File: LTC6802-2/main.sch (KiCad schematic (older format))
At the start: 10 parts, among them P1 CONN_01X13, P2 CONN_01X04, P3 CONN_01X04, P4 CONN_01X06, P5 CONN_01X13, U1 LTC6802-2

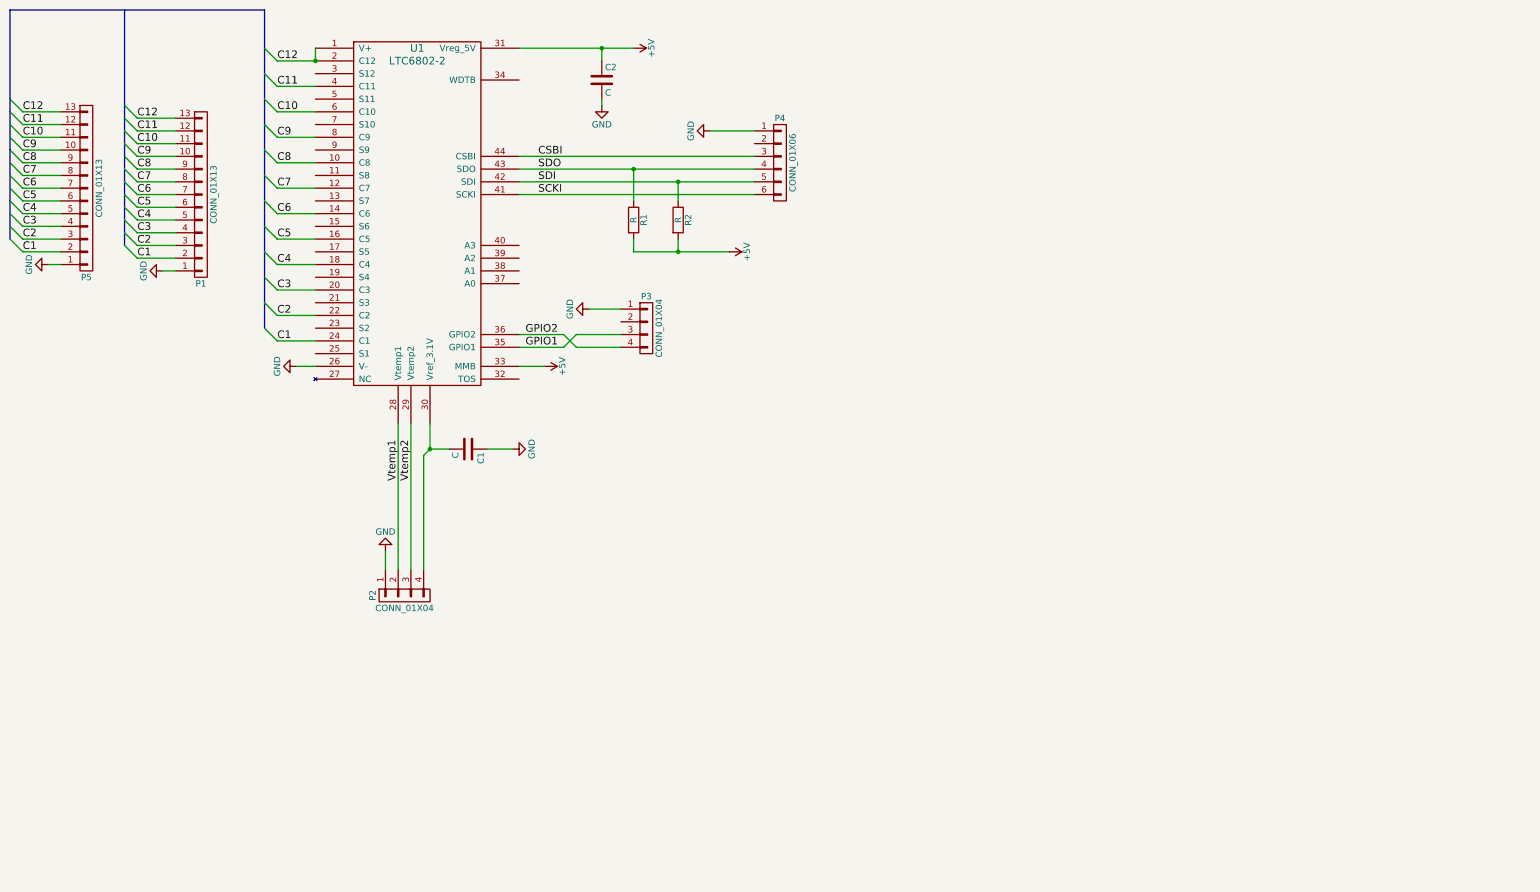
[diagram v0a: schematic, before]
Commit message: test
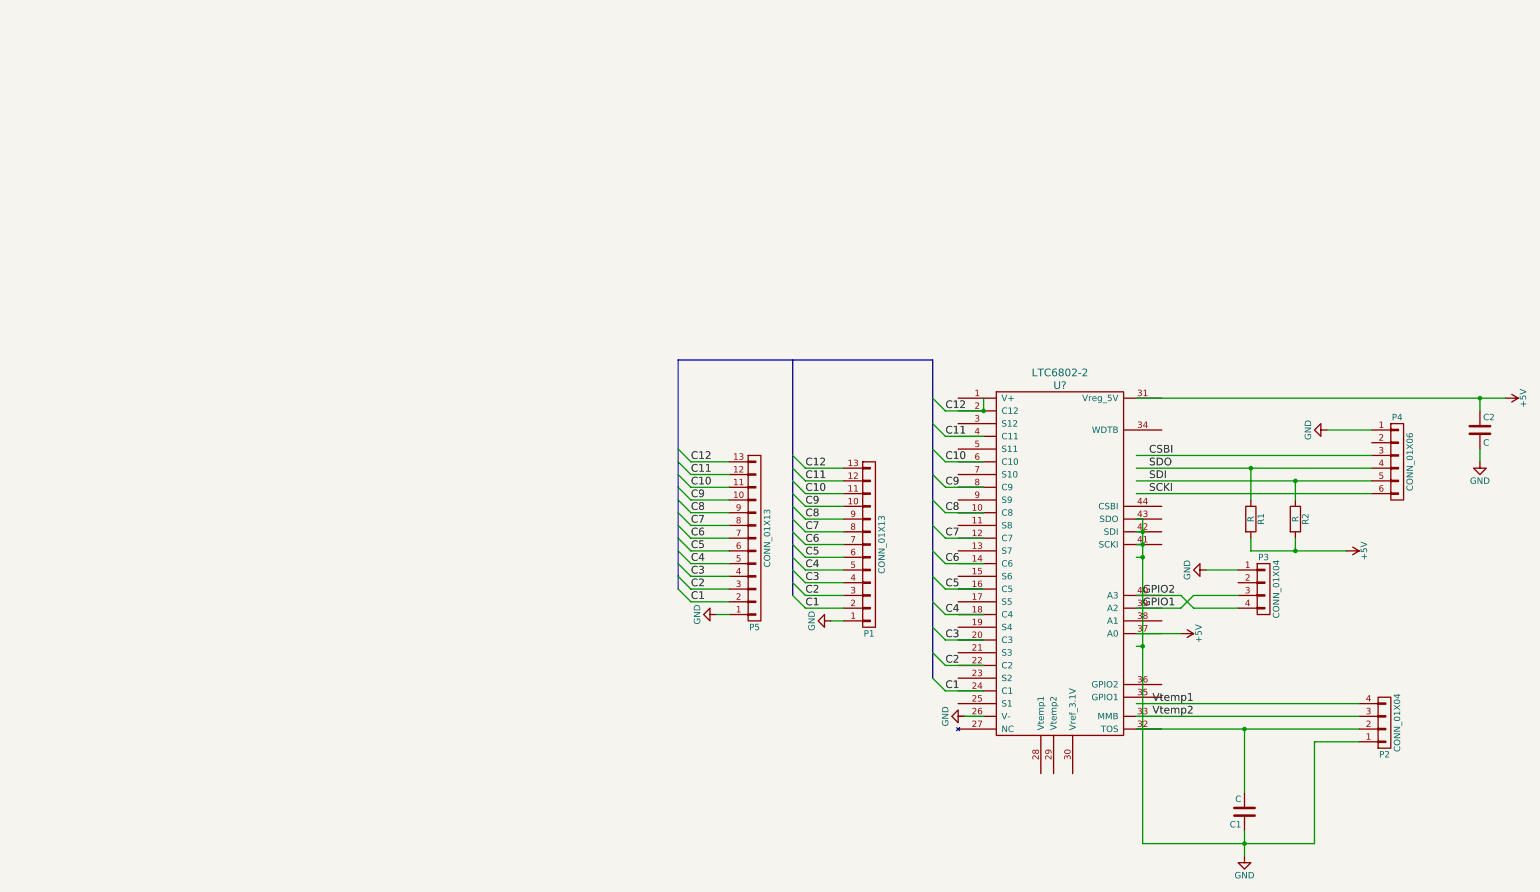
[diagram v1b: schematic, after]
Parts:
- removed U1: LTC6802-2, KiCad-Dev:SSOP-44, symbol LTC6802-2
- added U?: LTC6802-2, symbol LTC6802-2
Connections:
- wire segments 74 -> 75
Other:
- moved on the sheet: C1, C2, P1, P2, P3, P4, P5, R1, R2
